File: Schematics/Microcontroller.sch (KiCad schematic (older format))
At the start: 31 parts, among them IC2 STM32F730R8T6, J10 Conn_01x01, J11 Conn_01x01, J12 Conn_01x01, J13 Conn_01x01, J14 Conn_01x01, J15 Conn_01x01, J16 Conn_01x04, J19 Conn_01x01, J20 Conn_01x01, J21 Conn_01x01, J3 Conn_01x01, J8 Conn_01x01, J9 Conn_01x01, Y2 Crystal_GND23, Y3 Crystal_GND23

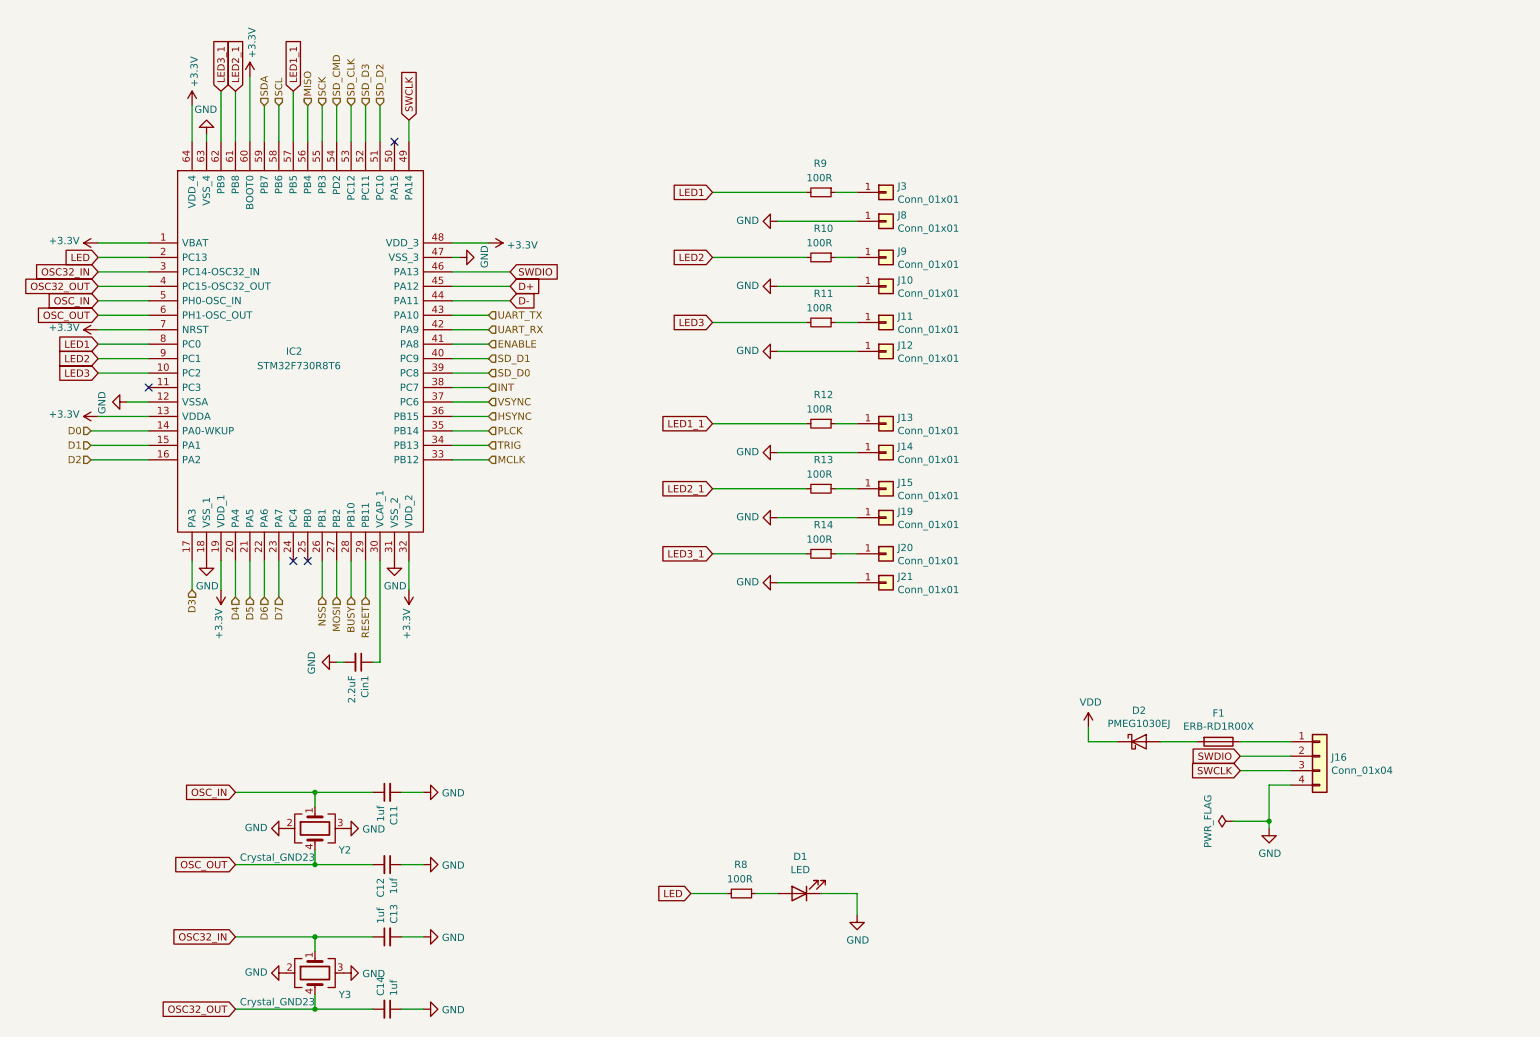
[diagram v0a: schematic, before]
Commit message: Add files via upload
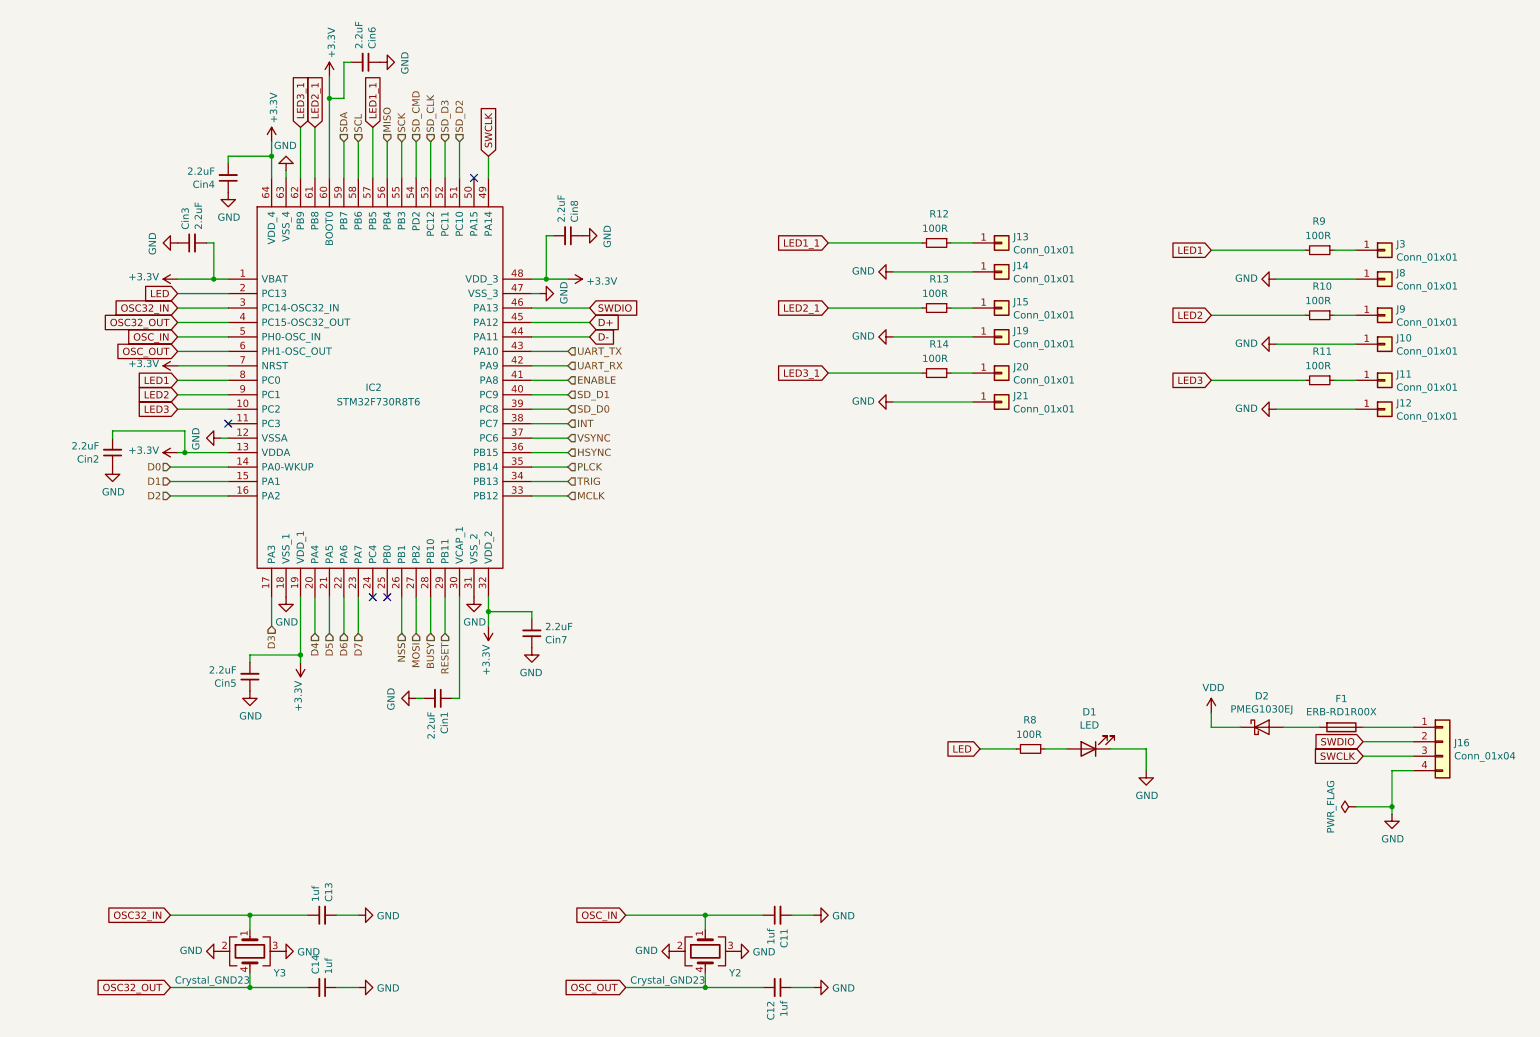
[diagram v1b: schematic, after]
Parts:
- added Cin2, Cin3, Cin4, Cin5, Cin6, Cin7, Cin8: 2.2uF, Capacitor_SMD:C_0402_1005Metric, symbol Device:C_Small
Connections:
- net +3V3: now also Cin2.2, Cin3.2, Cin4.2, Cin5.2, Cin6.2, Cin7.2, Cin8.2
- net GND: now also Cin2.1, Cin3.1, Cin4.1, Cin5.1, Cin6.1, Cin7.1, Cin8.1
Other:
- moved on the sheet: C11, C12, C13, C14, Cin1, D1, D2, F1, IC2, J10, J11, J12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
